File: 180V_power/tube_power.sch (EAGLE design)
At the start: 22 parts, among them IC1 NE555D, Q1 IRF740S, U1 TLV1117-5SOT-223, U2 2N7002

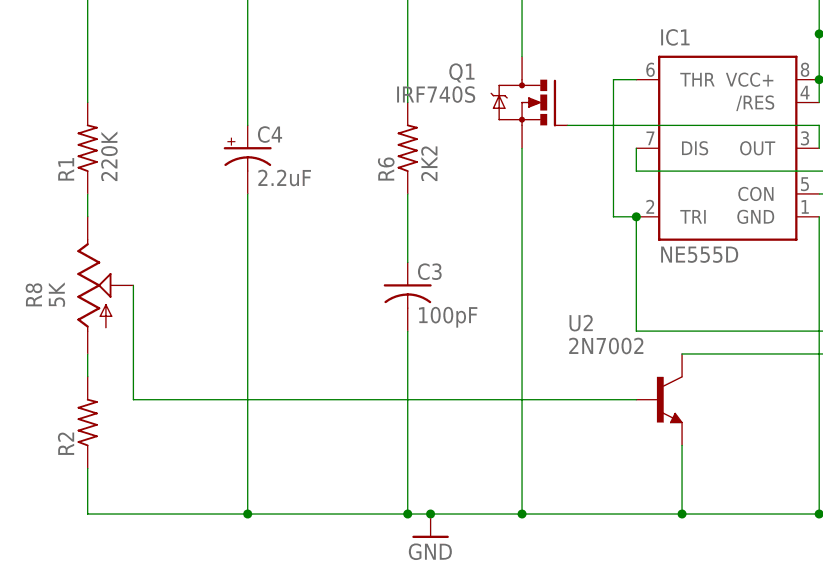
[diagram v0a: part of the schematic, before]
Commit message: update document data
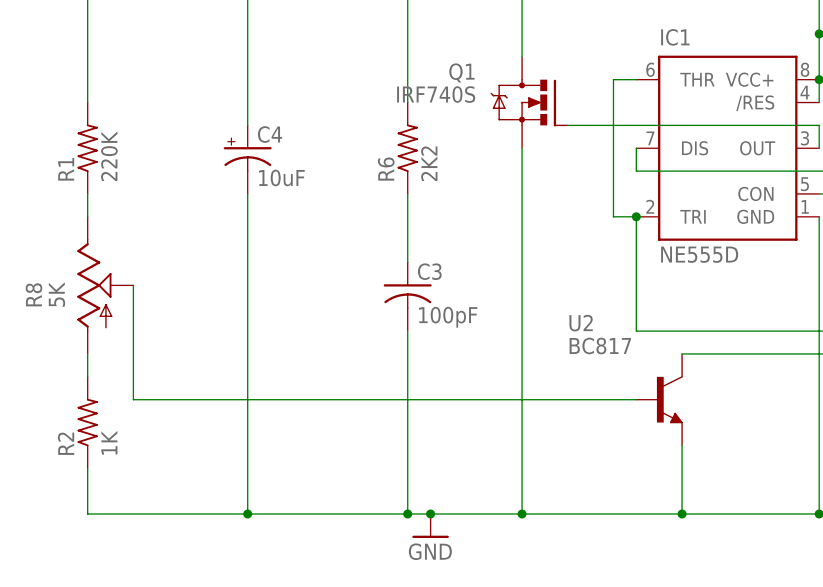
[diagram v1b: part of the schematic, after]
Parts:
- C4: value 2.2uF -> 10uF
- R2: value (none) -> 1K
- U2: value 2N7002 -> BC817
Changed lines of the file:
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@@
 <grid distance="0.1" unitdist="inch" unit="inch" style="lines" multiple="1" display="no" altdistance="0.01" altunitdist="inch" altunit="inch"/>
 <layers>
-<layer number="1" name="Top" color="4" fill="1" visible="yes" active="no"/>
-<layer number="2" name="Route2" color="1" fill="3" visible="yes" active="no"/>
-<layer number="3" name="Route3" color="4" fill="3" visible="yes" active="no"/>
-<layer number="4" name="Route4" color="1" fill="4" visible="yes" active="no"/>
-<layer number="5" name="Route5" color="4" fill="4" visible="yes" active="no"/>
-<layer number="6" name="Route6" color="1" fill="8" visible="yes" active="no"/>
-<layer number="7" name="Route7" color="4" fill="8" visible="yes" active="no"/>
-<layer number="8" name="Route8" color="1" fill="2" visible="yes" active="no"/>
-<layer number="9" name="Route9" color="4" fill="2" visible="yes" active="no"/>
-<layer number="10" name="Route10" color="1" fill="7" visible="yes" active="no"/>
-<layer number="11" name="Route11" color="4" fill="7" visible="yes" active="no"/>
-<layer number="12" name="Route12" color="1" fill="5" visible="yes" active="no"/>
-<layer number="13" name="Route13" color="4" fill="5" visible="yes" active="no"/>
-<layer number="14" name="Route14" color="1" fill="6" visible="yes" active="no"/>
-<layer number="15" name="Route15" color="4" fill="6" visible="yes" active="no"/>
-<layer number="16" name="Bottom" color="1" fill="1" visible="yes" active="no"/>
-<layer number="17" name="Pads" color="2" fill="1" visible="yes" active="no"/>
-<layer number="18" name="Vias" color="2" fill="1" visible="yes" active="no"/>
-<layer number="19" name="Unrouted" color="6" fill="1" visible="yes" active="no"/>
-<layer number="20" name="Dimension" color="15" fill="1" visible="yes" active="no"/>
-<layer number="21" name="tPlace" color="7" fill="1" visible="yes" active="no"/>
-<layer number="22" name="bPlace" color="7" fill="1" visible="yes" active="no"/>
-<layer number="23" name="tOrigins" color="15" fill="1" visible="yes" active="no"/>
-<layer number="24" name="bOrigins" color="15" fill="1" visible="yes" active="no"/>
-<layer number="25" name="tNames" color="7" fill="1" visible="yes" active="no"/>
-<layer number="26" name="bNames" color="7" fill="1" visible="yes" active="no"/>
-<layer number="27" name="tValues" color="6" fill="1" visible="yes" active="no"/>
-<layer number="28" name="bValues" color="5" fill="1" visible="yes" active="no"/>
+<layer number="1" name="Top" color="4" fill="1" visible="no" active="no"/>
+<layer number="2" name="Route2" color="1" fill="3" visible="no" active="no"/>
+<layer number="3" name="Route3" color="4" fill="3" visible="no" active="no"/>
+<layer number="4" name="Route4" color="1" fill="4" visible="no" active="no"/>
+<layer number="5" name="Route5" color="4" fill="4" visible="no" active="no"/>
+<layer number="6" name="Route6" color="1" fill="8" visible="no" active="no"/>
+<layer number="7" name="Route7" color="4" fill="8" visible="no" active="no"/>
+<layer number="8" name="Route8" color="1" fill="2" visible="no" active="no"/>
+<layer number="9" name="Route9" color="4" fill="2" visible="no" active="no"/>
+<layer number="10" name="Route10" color="1" fill="7" visible="no" active="no"/>
+<layer number="11" name="Route11" color="4" fill="7" visible="no" active="no"/>
+<layer number="12" name="Route12" color="1" fill="5" visible="no" active="no"/>
+<layer number="13" name="Route13" color="4" fill="5" visible="no" active="no"/>
+<layer number="14" name="Route14" color="1" fill="6" visible="no" active="no"/>
+<layer number="15" name="Route15" color="4" fill="6" visible="no" active="no"/>
+<layer number="16" name="Bottom" color="1" fill="1" visible="no" active="no"/>
+<layer number="17" name="Pads" color="2" fill="1" visible="no" active="no"/>
+<layer number="18" name="Vias" color="2" fill="1" visible="no" active="no"/>
+<layer number="19" name="Unrouted" color="6" fill="1" visible="no" active="no"/>
+<layer number="20" name="Dimension" color="15" fill="1" visible="no" active="no"/>
+<layer number="21" name="tPlace" color="7" fill="1" visible="no" active="no"/>
+<layer number="22" name="bPlace" color="7" fill="1" visible="no" active="no"/>
+<layer number="23" name="tOrigins" color="15" fill="1" visible="no" active="no"/>
+<layer number="24" name="bOrigins" color="15" fill="1" visible="no" active="no"/>
+<layer number="25" name="tNames" color="7" fill="1" visible="no" active="no"/>
+<layer number="26" name="bNames" color="7" fill="1" visible="no" active="no"/>
+<layer number="27" name="tValues" color="6" fill="1" visible="no" active="no"/>
+<layer number="28" name="bValues" color="5" fill="1" visible="no" active="no"/>
 <layer number="29" name="tStop" color="7" fill="3" visible="no" active="no"/>
 <layer number="30" name="bStop" color="7" fill="6" visible="no" active="no"/>
@@
 <layer number="35" name="tGlue" color="7" fill="4" visible="no" active="no"/>
 <layer number="36" name="bGlue" color="7" fill="5" visible="no" active="no"/>
-<layer number="37" name="tTest" color="7" fill="1" visible="yes" active="no"/>
-<layer number="38" name="bTest" color="7" fill="1" visible="yes" active="no"/>
+<layer number="37" name="tTest" color="7" fill="1" visible="no" active="no"/>
+<layer number="38" name="bTest" color="7" fill="1" visible="no" active="no"/>
 <layer number="39" name="tKeepout" color="4" fill="11" visible="no" active="no"/>
 <layer number="40" name="bKeepout" color="1" fill="11" visible="no" active="no"/>
@@
 <layer number="44" name="Drills" color="7" fill="1" visible="no" active="no"/>
 <layer number="45" name="Holes" color="7" fill="1" visible="no" active="no"/>
-<layer number="46" name="Milling" color="3" fill="1" visible="yes" active="no"/>
-<layer number="47" name="Measures" color="7" fill="1" visible="yes" active="no"/>
-<layer number="48" name="Document" color="7" fill="1" visible="yes" active="no"/>
-<layer number="49" name="Reference" color="7" fill="1" visible="yes" active="no"/>
-<layer number="50" name="dxf" color="7" fill="1" visible="yes" active="no"/>
-<layer number="51" name="tDocu" color="7" fill="1" visible="yes" active="no"/>
-<layer number="52" name="bDocu" color="7" fill="1" visible="yes" active="no"/>
-<layer number="53" name="tGND_GNDA" color="7" fill="9" visible="yes" active="no"/>
-<layer number="54" name="bGND_GNDA" color="1" fill="9" visible="yes" active="no"/>
-<layer number="56" name="wert" color="7" fill="1" visible="yes" active="no"/>
+<layer number="46" name="Milling" color="3" fill="1" visible="no" active="no"/>
+<layer number="47" name="Measures" color="7" fill="1" visible="no" active="no"/>
+<layer number="48" name="Document" color="7" fill="1" visible="no" active="no"/>
+<layer number="49" name="Reference" color="7" fill="1" visible="no" active="no"/>
+<layer number="50" name="dxf" color="7" fill="1" visible="no" active="no"/>
+<layer number="51" name="tDocu" color="7" fill="1" visible="no" active="no"/>
+<layer number="52" name="bDocu" color="7" fill="1" visible="no" active="no"/>
+<layer number="53" name="tGND_GNDA" color="7" fill="9" visible="no" active="no"/>
+<layer number="54" name="bGND_GNDA" color="1" fill="9" visible="no" active="no"/>
+<layer number="56" name="wert" color="7" fill="1" visible="no" active="no"/>
 <layer number="91" name="Nets" color="2" fill="1" visible="yes" active="yes"/>
 <layer number="92" name="Busses" color="1" fill="1" visible="yes" active="yes"/>
@@
 <part name="IC1" library="iStivi - ICs" deviceset="NE555" device="D" value="NE555D"/>
 <part name="D1" library="iStivi - RCLD" deviceset="DIODE" device="SMA" value="1N4007"/>
-<part name="C4" library="iStivi - RCLD" deviceset="CAPACITOR_POL" device="E3.5-8" value="2.2uF"/>
+<part name="C4" library="iStivi - RCLD" deviceset="CAPACITOR_POL" device="E3.5-8" value="10uF"/>
 <part name="C1" library="iStivi - RCLD" deviceset="CAPACITOR_POL" device="E5-10.5" value="330uF"/>
 <part name="R5" library="iStivi - RCLD" deviceset="RESISTOR" device="R0805" value="56K"/>
@@
 <part name="C5" library="iStivi - RCLD" deviceset="CAPACITOR_POL" device="E2-5" value="10uF"/>
 <part name="U1" library="iStivi - Transistor-FET-reg" deviceset="TLV1117-5" device="SOT-223"/>
-<part name="U2" library="iStivi - Transistor-FET-reg" deviceset="BC817" device="" value="2N7002"/>
+<part name="U2" library="iStivi - Transistor-FET-reg" deviceset="BC817" device="" value="BC817"/>
 <part name="L1" library="iStivi - RCLD" deviceset="INDUCTOR" device="" value="180uH"/>
 <part name="Q1" library="iStivi - Transistor-FET-reg" deviceset="IRF740" device="S"/>
@@
 <part name="R8" library="iStivi - RCLD" deviceset="TRIM_POT" device="EVM2N" value="5K"/>
 <part name="D2" library="iStivi - RCLD" deviceset="DIODE" device="SOD-80"/>
-<part name="R2" library="iStivi - RCLD" deviceset="RESISTOR" device="R1206"/>
+<part name="R2" library="iStivi - RCLD" deviceset="RESISTOR" device="R1206" value="1K"/>
 </parts>
 <sheets>
